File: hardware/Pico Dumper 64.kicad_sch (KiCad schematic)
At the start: 6 parts, among them J1 N64_Slot, J2 Conn_01x01, J3 Conn_01x01, J4 Conn_01x01, U1 Pico

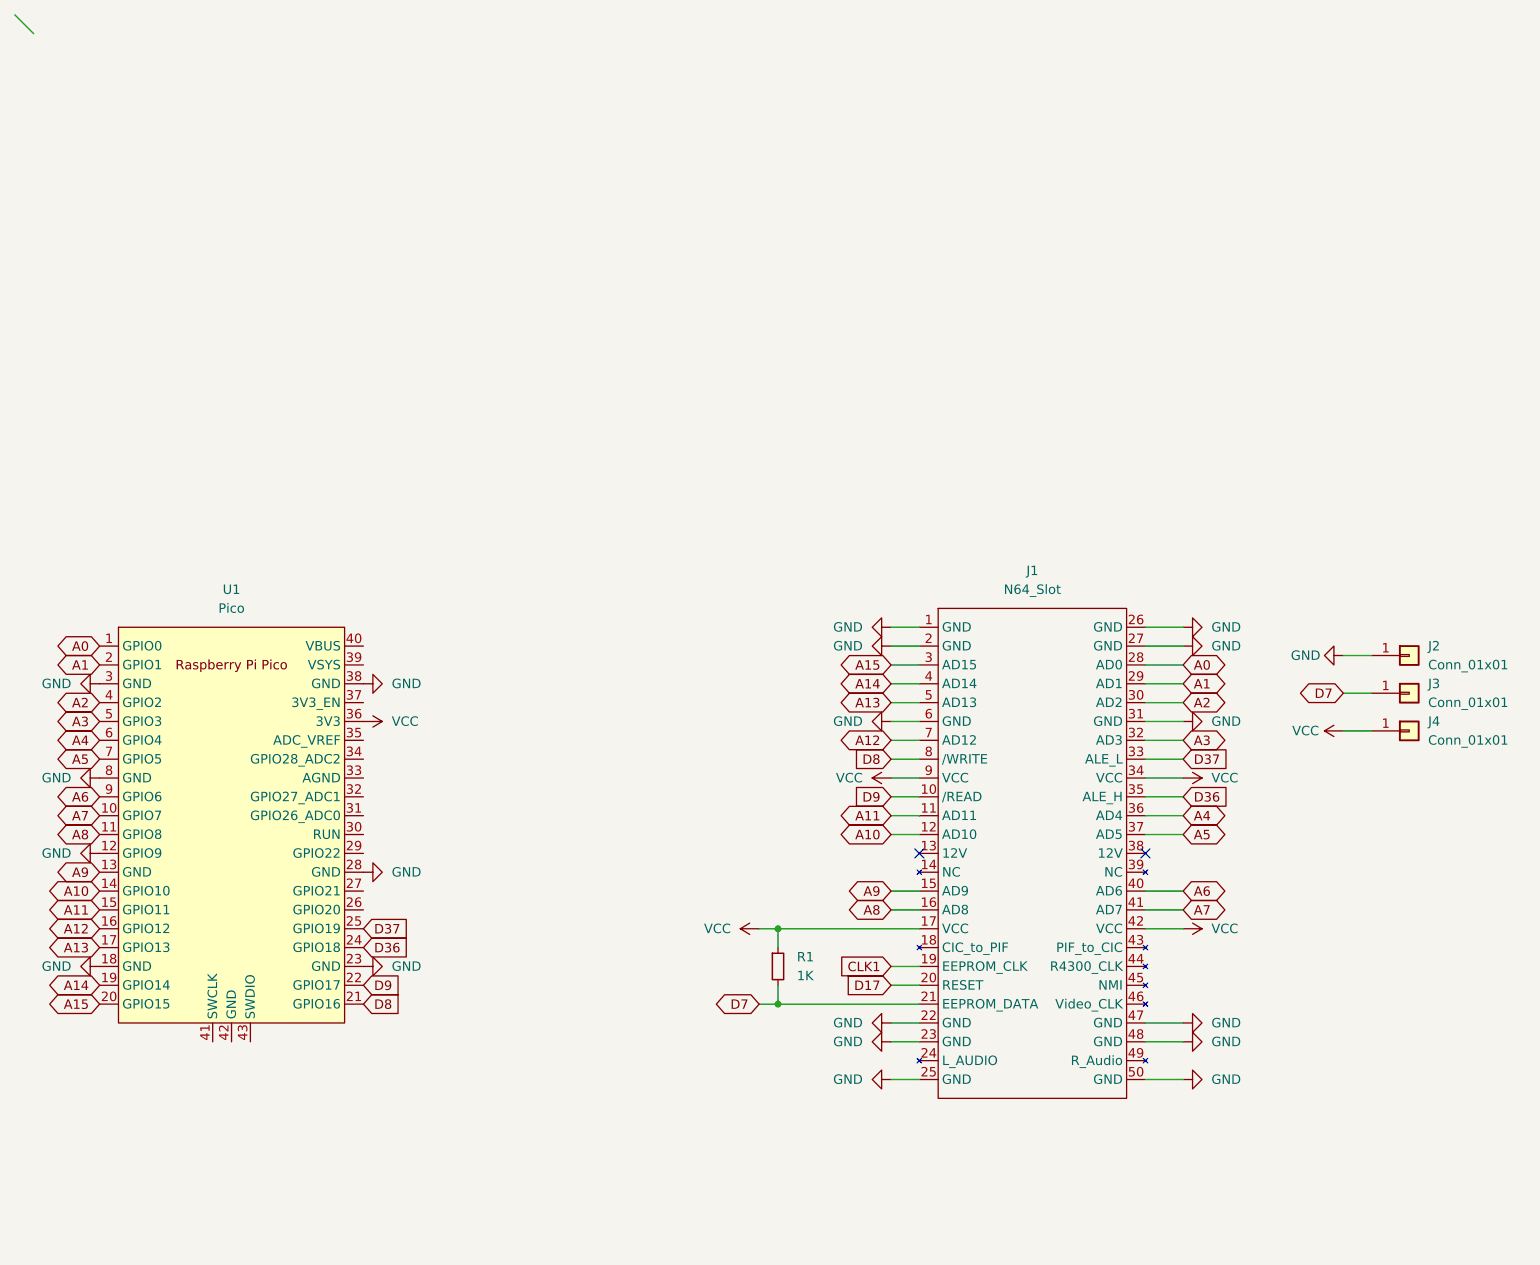
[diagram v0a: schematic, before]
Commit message: update sch
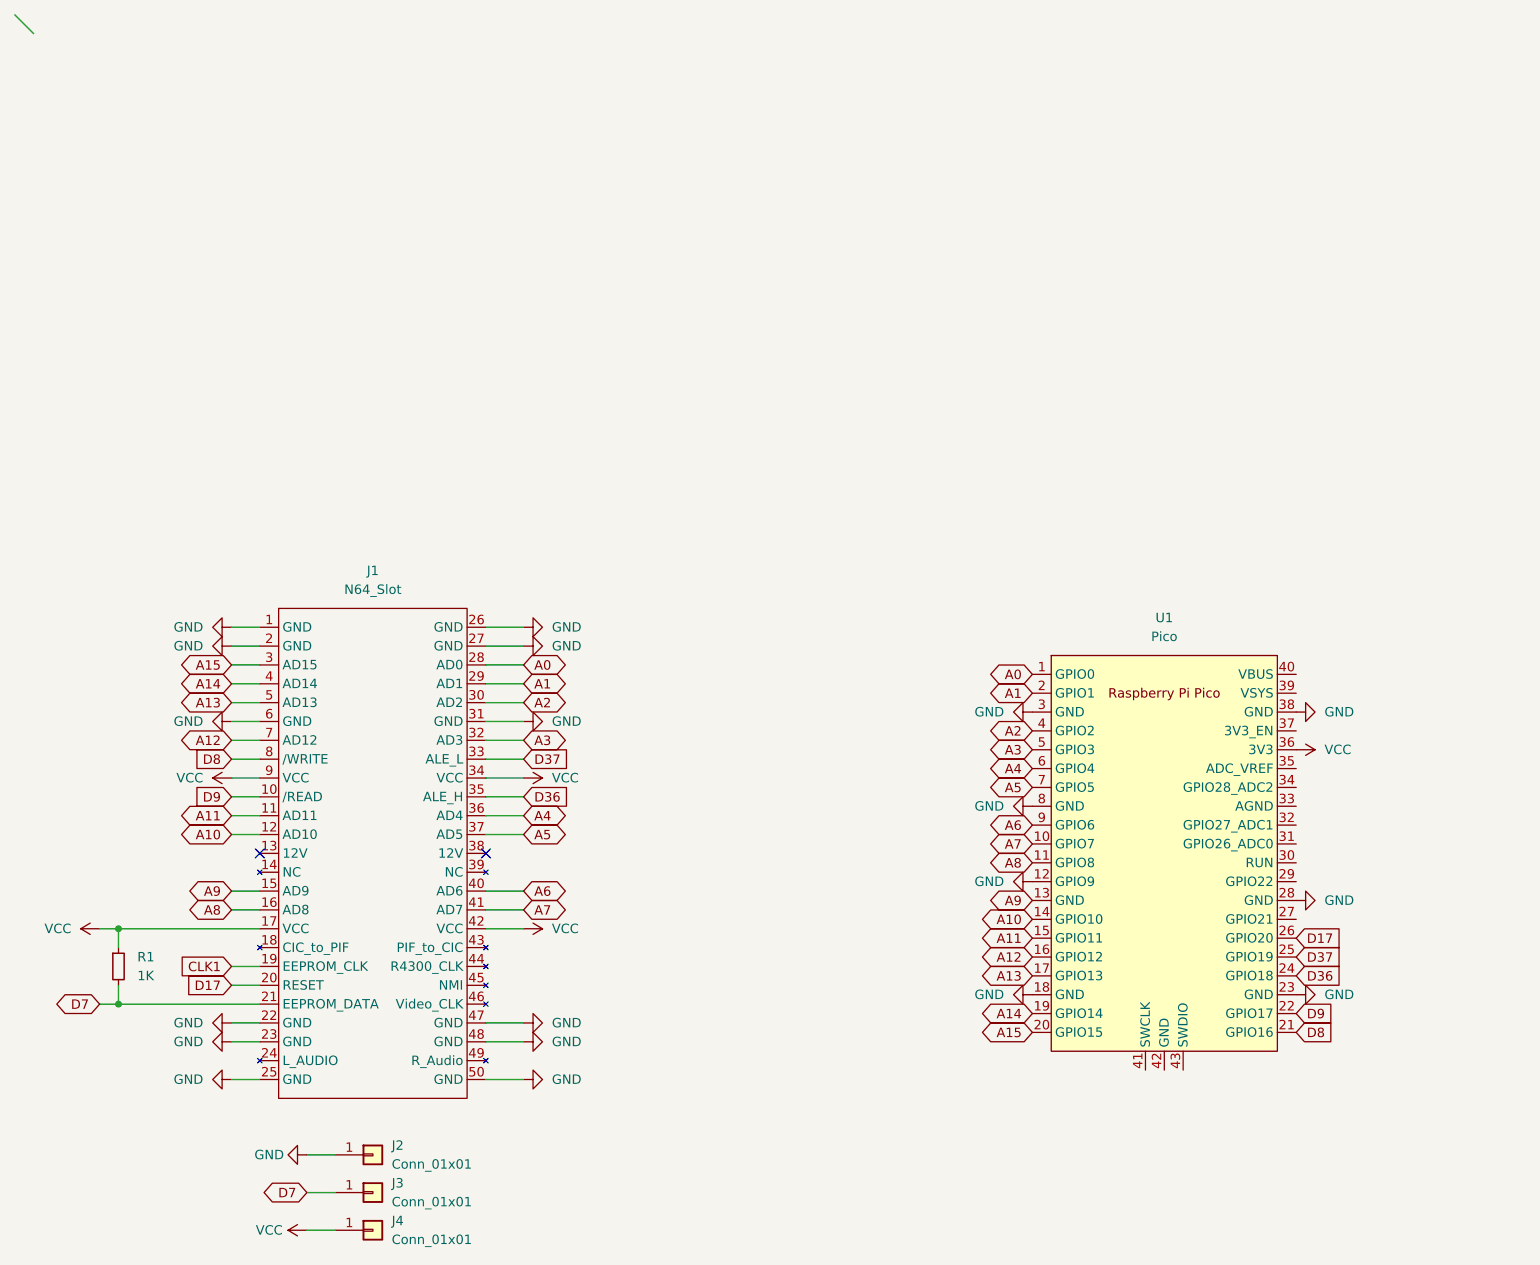
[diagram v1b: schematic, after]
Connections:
- net D17: now also U1.26 (GPIO20)
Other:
- moved on the sheet: J1, J2, J3, J4, R1, U1
